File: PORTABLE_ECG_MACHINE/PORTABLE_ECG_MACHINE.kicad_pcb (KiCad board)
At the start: 2 copper layers, 25.5 x 64.8 mm, 79 parts, among them IC1 AD8232ACPZ, J1 UART, J2 AudioJack3, J3 Li-Ion 3.7 CONN, J4 USB_C_Receptacle_USB2.0, Q1 BSS138, Q2 BSS138, SW1 SW_SPDT, U1 SSD1306, U2 CP2102-GM, U3 TC1262-33, U4 TP4056

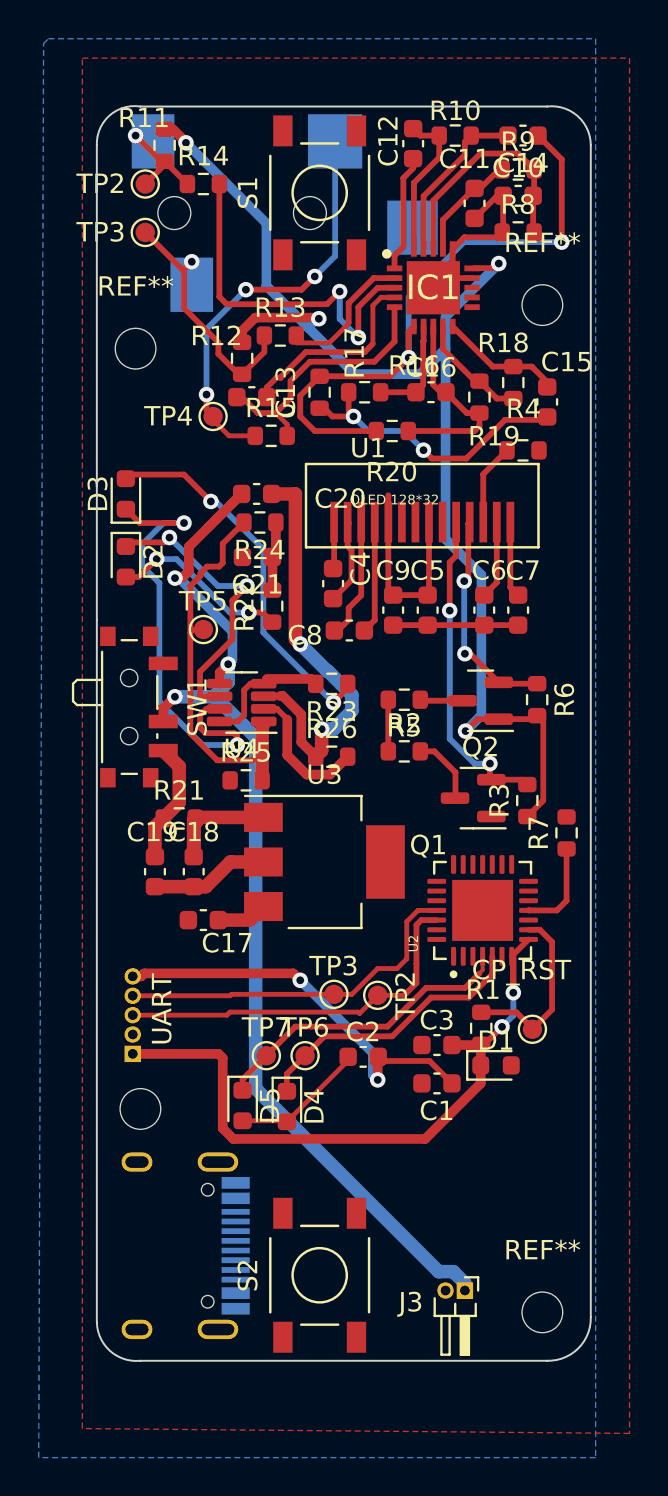
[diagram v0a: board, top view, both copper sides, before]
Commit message: DRC CHECK
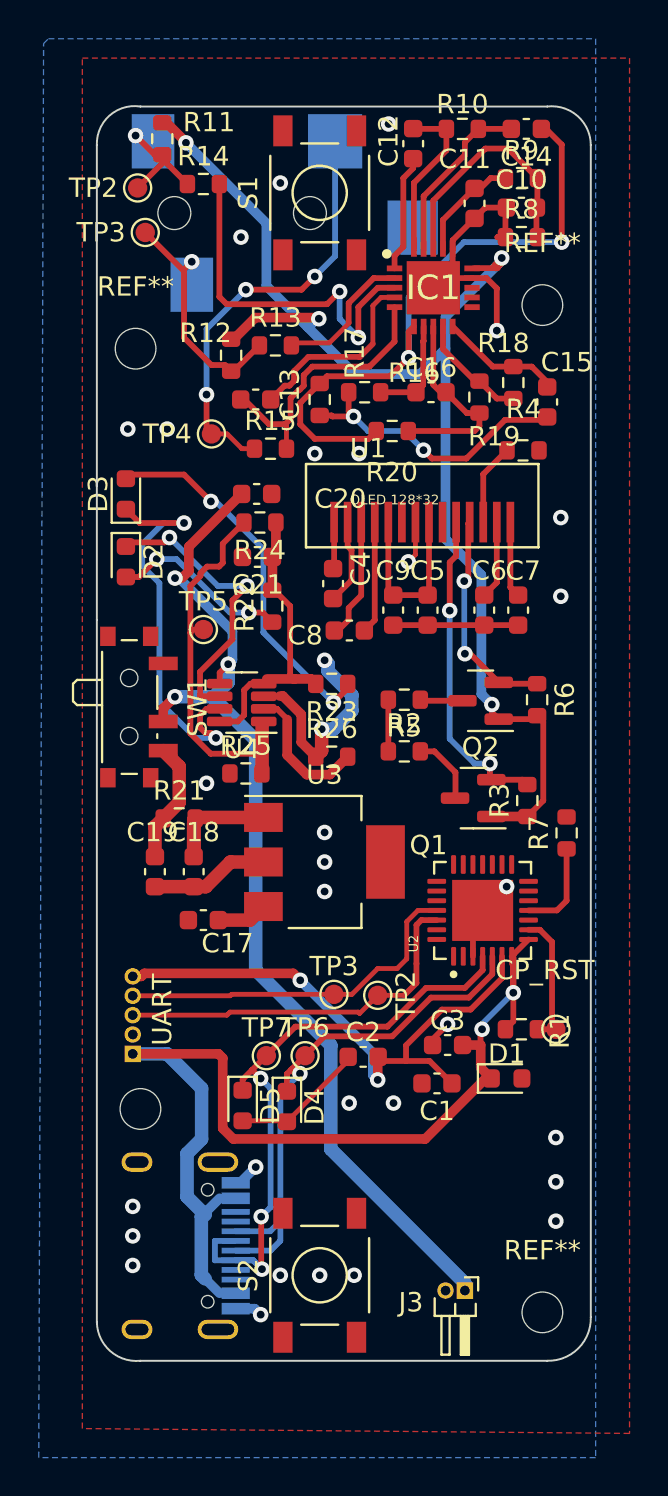
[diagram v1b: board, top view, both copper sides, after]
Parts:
- moved R1 2.07 mm to (105.9, 72.1), turned to 0 degrees
- moved CP_RST 1.21 mm to (107.7, 72.1)
- moved TP4 0.91 mm to (89.9, 41.4)
- moved D1 0.87 mm to (105.2, 74.7)
- moved R15 0.66 mm to (93.0, 42.2)
- moved C10 0.63 mm to (105.9, 29.7)
- moved R12 0.59 mm to (90.9, 37.3)
- moved R13 0.57 mm to (93.2, 36.8)
- moved C3 0.55 mm to (102.1, 72.9)
- moved R10 0.51 mm to (102.9, 25.7)
- moved R9 0.47 mm to (105.9, 28.2)
- moved TP2 0.44 mm to (86.1, 28.7)
- moved C14 0.39 mm to (106.2, 25.7)
- moved R16 0.37 mm to (95.5, 39.6)
- moved R11 0.36 mm to (87.4, 26.2)
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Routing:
- net VIN: track 35.2 -> 56.1 mm
- net USB_D-: track 16.0 -> 33.2 mm, vias 0 -> 3
- net USB_D+: track 14.6 -> 29.2 mm, vias 0 -> 1
- net Net-(C1-Pad1): track 21.5 -> 29.6 mm
- net Net-(C21-Pad1): track 10.0 -> 15.2 mm
- net /BATTERY +VE: track 59.5 -> 56.6 mm
- net Net-(D3-Pad1): track 23.7 -> 20.9 mm
- net Net-(R1-Pad2): track 9.34 -> 7.02 mm
- net Net-(C5-Pad2): track 11.0 -> 9.58 mm
- net GND: track 53.1 -> 54.4 mm, vias 2 -> 32
- net Net-(C14-Pad1): track 31.3 -> 32.4 mm
- net /LA: track 5.30 -> 6.08 mm
- net Net-(C12-Pad2): track 7.89 -> 8.62 mm
- net Net-(R24-Pad2): track 20.6 -> 19.9 mm
- net /RL: track 21.5 -> 22.2 mm
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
